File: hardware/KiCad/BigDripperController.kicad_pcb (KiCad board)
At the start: 4 copper layers, 209.1 x 208.6 mm, 95 parts, among them Q1 IRL540NPBF, Q10 IRL540NPBF, Q11 IRL540NPBF, Q12 IRL540NPBF, Q13 IRL540NPBF, Q14 IRL540NPBF, Q15 IRL540NPBF, Q16 IRL540NPBF, Q17 TL2575-05IKV, Q2 IRL540NPBF, Q3 IRL540NPBF, Q4 IRL540NPBF, Q5 IRL540NPBF, Q6 IRL540NPBF, Q7 IRL540NPBF, Q8 IRL540NPBF, Q9 IRL540NPBF, U18 SN74HCT125NE4, U2 SN74HCT125NE4, U3 SN74HCT125NE4, U4 SN74HCT125NE4, U5 SN74HCT125NE4

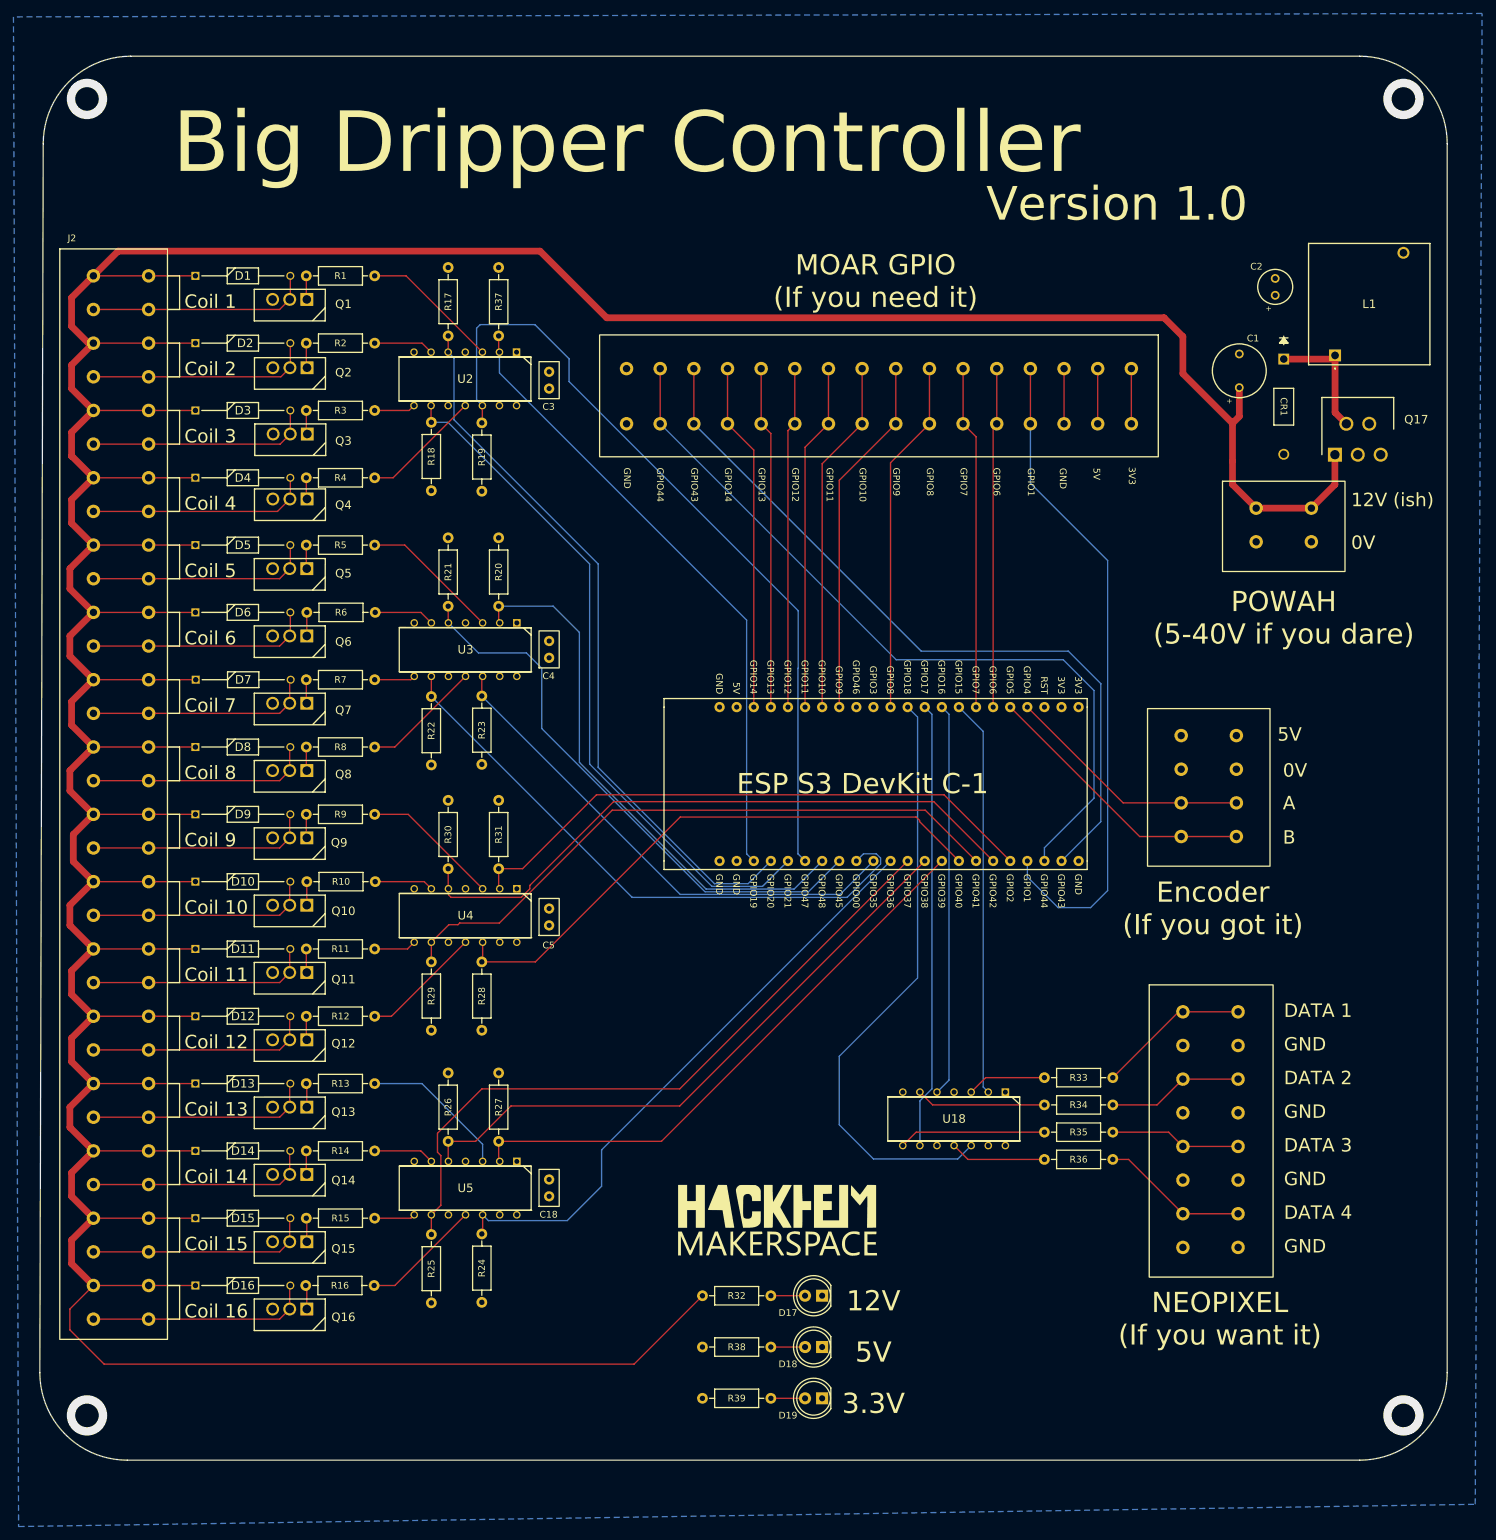
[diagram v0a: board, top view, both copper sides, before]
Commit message: Added updated schematic and layout.
* Added production files for 1.1
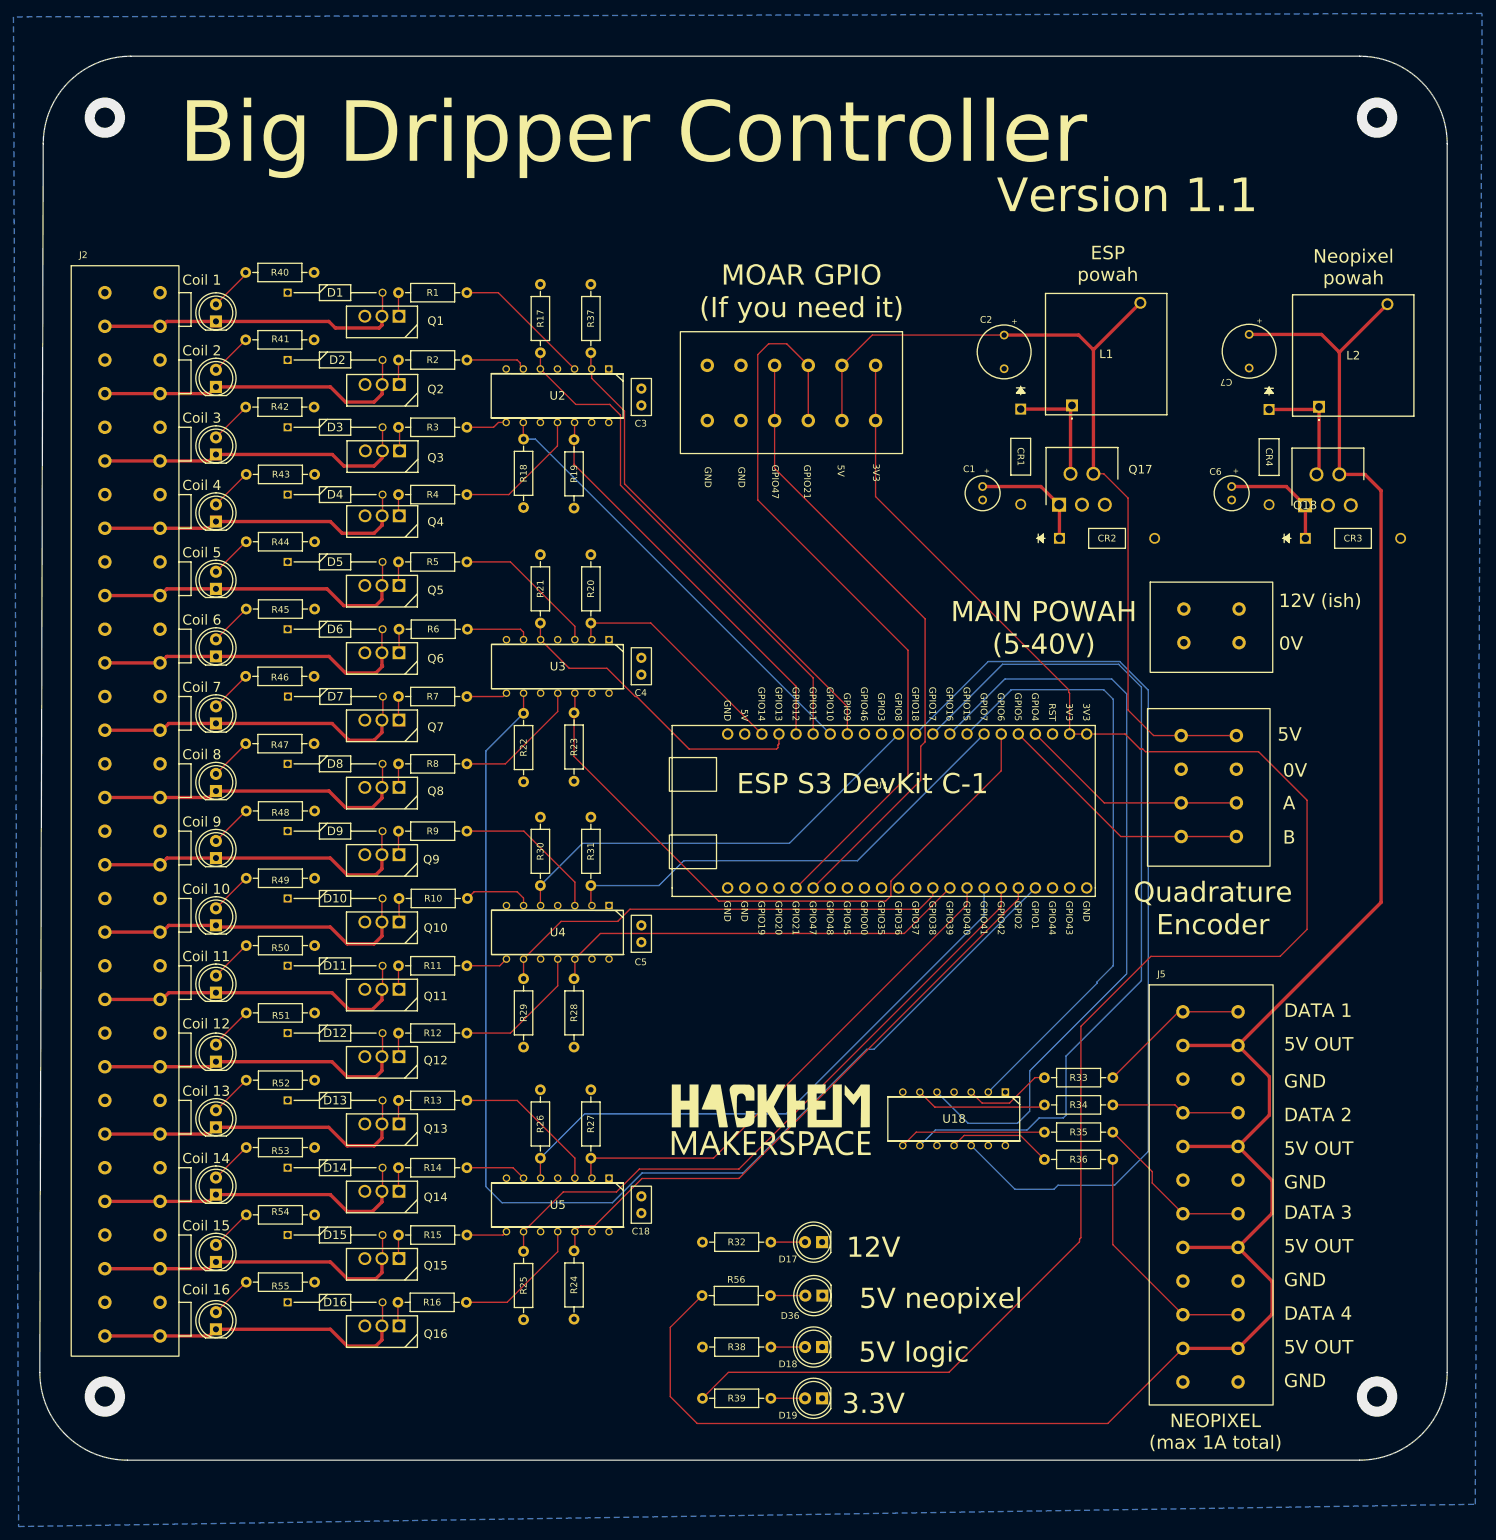
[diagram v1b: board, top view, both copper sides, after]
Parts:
- added C6: 100uF, hackheim:CAP ALUM 10UF 20% 25V RADIAL TH - WÜRTH - 860020472003, F.Cu at (223.4, 40.8)
- added C7: 330uF, hackheim:CAP ALUM 10UF 20% 25V RADIAL TH - WÜRTH - 860020472003, F.Cu at (226.5, 18.2)
- added CR2: 1N5819, hackheim:DO-41_STM, F.Cu at (197.8, 47.5)
- added CR3: 1N5819, hackheim:DO-41_STM, F.Cu at (234.4, 47.5)
- added CR4: 1N5819, hackheim:DO-41_STM, F.Cu at (229.0, 28.4)
- added D20: LED, LED_THT:LED_D5.0mm, F.Cu at (72.5, 15.3)
- added D21: LED, LED_THT:LED_D5.0mm, F.Cu at (72.5, 25.0)
- added D22: LED, LED_THT:LED_D5.0mm, F.Cu at (72.5, 35.0)
- added D23: LED, LED_THT:LED_D5.0mm, F.Cu at (72.5, 45.0)
- added D24: LED, LED_THT:LED_D5.0mm, F.Cu at (72.5, 55.0)
- added D25: LED, LED_THT:LED_D5.0mm, F.Cu at (72.5, 65.0)
- added D26: LED, LED_THT:LED_D5.0mm, F.Cu at (72.5, 75.0)
- added D27: LED, LED_THT:LED_D5.0mm, F.Cu at (72.5, 85.0)
- added D28: LED, LED_THT:LED_D5.0mm, F.Cu at (72.5, 95.0)
- added D29: LED, LED_THT:LED_D5.0mm, F.Cu at (72.5, 105.0)
- added D30: LED, LED_THT:LED_D5.0mm, F.Cu at (72.5, 115.0)
- added D31: LED, LED_THT:LED_D5.0mm, F.Cu at (72.5, 125.2)
- added D32: LED, LED_THT:LED_D5.0mm, F.Cu at (72.5, 135.0)
- added D33: LED, LED_THT:LED_D5.0mm, F.Cu at (72.5, 145.0)
- added D34: LED, LED_THT:LED_D5.0mm, F.Cu at (72.5, 155.0)
- added D35: LED, LED_THT:LED_D5.0mm, F.Cu at (72.5, 165.0)
- added D36: LED, LED_THT:LED_D5.0mm, F.Cu at (162.6, 160.0)
- added L2: PE-52627NL, hackheim:PE52627NL, F.Cu at (236.4, 28.0)
- added Q18: TL2575-05IKV, hackheim:TL2575-05IKV, F.Cu at (234.3, 42.6)
- added R40: 2k, Resistor_THT:R_Axial_DIN0207_L6.3mm_D2.5mm_P10.16mm_Horizontal, F.Cu at (87.1, 8.00)
- added R41: 2k, Resistor_THT:R_Axial_DIN0207_L6.3mm_D2.5mm_P10.16mm_Horizontal, F.Cu at (87.1, 18.0)
- added R42: 2k, Resistor_THT:R_Axial_DIN0207_L6.3mm_D2.5mm_P10.16mm_Horizontal, F.Cu at (87.1, 28.0)
- added R43: 2k, Resistor_THT:R_Axial_DIN0207_L6.3mm_D2.5mm_P10.16mm_Horizontal, F.Cu at (87.2, 38.0)
- added R44: 2k, Resistor_THT:R_Axial_DIN0207_L6.3mm_D2.5mm_P10.16mm_Horizontal, F.Cu at (87.2, 48.0)
- added R45: 2k, Resistor_THT:R_Axial_DIN0207_L6.3mm_D2.5mm_P10.16mm_Horizontal, F.Cu at (87.2, 58.0)
- added R46: 2k, Resistor_THT:R_Axial_DIN0207_L6.3mm_D2.5mm_P10.16mm_Horizontal, F.Cu at (87.1, 68.0)
- added R47: 2k, Resistor_THT:R_Axial_DIN0207_L6.3mm_D2.5mm_P10.16mm_Horizontal, F.Cu at (87.1, 78.0)
- added R48: 2k, Resistor_THT:R_Axial_DIN0207_L6.3mm_D2.5mm_P10.16mm_Horizontal, F.Cu at (87.2, 88.0)
- added R49: 2k, Resistor_THT:R_Axial_DIN0207_L6.3mm_D2.5mm_P10.16mm_Horizontal, F.Cu at (87.2, 98.0)
- added R50: 2k, Resistor_THT:R_Axial_DIN0207_L6.3mm_D2.5mm_P10.16mm_Horizontal, F.Cu at (87.2, 108.0)
- added R51: 2k, Resistor_THT:R_Axial_DIN0207_L6.3mm_D2.5mm_P10.16mm_Horizontal, F.Cu at (87.2, 118.0)
- added R52: 2k, Resistor_THT:R_Axial_DIN0207_L6.3mm_D2.5mm_P10.16mm_Horizontal, F.Cu at (87.2, 128.0)
- added R53: 2k, Resistor_THT:R_Axial_DIN0207_L6.3mm_D2.5mm_P10.16mm_Horizontal, F.Cu at (87.2, 138.0)
- added R54: 2k, Resistor_THT:R_Axial_DIN0207_L6.3mm_D2.5mm_P10.16mm_Horizontal, F.Cu at (87.2, 148.0)
- added R55: 2k, Resistor_THT:R_Axial_DIN0207_L6.3mm_D2.5mm_P10.16mm_Horizontal, F.Cu at (87.2, 158.0)
- added R56: R, Resistor_THT:R_Axial_DIN0207_L6.3mm_D2.5mm_P10.16mm_Horizontal, F.Cu at (144.7, 160.0)
- moved C1 43.4 mm to (186.4, 40.8), turned to 90 degrees
- moved C2 42.7 mm to (188.6, 19.8), turned to 90 degrees
- moved Q17 41.6 mm to (197.8, 42.5)
- moved CR1 39.8 mm to (192.1, 28.3)
- moved L1 39.8 mm to (199.7, 27.8)
- moved J4 38.0 mm to (170.5, 21.8)
- moved J1 18.4 mm to (216.3, 58.0)
- moved REF** 14.9 mm to (154.0, 132.4)
- moved R19 13.9 mm to (125.7, 32.8)
- moved D1 13.9 mm to (83.2, 11.0)
- moved D10 13.9 mm to (83.2, 101.0)
- moved D11 13.9 mm to (83.2, 111.0)
- moved D12 13.9 mm to (83.2, 121.0)
- moved D13 13.9 mm to (83.2, 131.0)
- moved D14 13.9 mm to (83.2, 141.0)
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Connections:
- net Net-(D1-A) renamed C1
- net Net-(D10-A) renamed C10
- net Net-(D11-A) renamed C11
- net Net-(D12-A) renamed C12
- net Net-(D13-A) renamed C13
- net Net-(D14-A) renamed C14
- net Net-(D15-A) renamed C15
- net Net-(D16-A) renamed C16
- net Net-(D2-A) renamed C2
- net Net-(D3-A) renamed C3
- net Net-(D4-A) renamed C4
- net Net-(D5-A) renamed C5
- net Net-(D6-A) renamed C6
- net Net-(D7-A) renamed C7
- net Net-(D8-A) renamed C8
- net Net-(D9-A) renamed C9
- C1 pad 1: 12V -> Net-(Q17-VIN)
- J4 pad 3: GND -> GPIO21
- J4 pad 4: GPIO1 -> GPIO47
- J4 pad 5: GPIO6 -> GND
- J4 pad 6: GPIO7 -> GND
- Q17 pad 1: 12V -> Net-(Q17-VIN)
- U1 pad 12: GPIO8 -> COIL15
- U1 pad 15: GPIO9 -> COIL1
- U1 pad 16: GPIO10 -> COIL3
- U1 pad 17: GPIO11 -> COIL2
- U1 pad 18: GPIO12 -> COIL4
- U1 pad 19: GPIO13 -> COIL6
- U1 pad 20: GPIO14 -> COIL5
- U1 pad 25: COIL1 -> unconnected-(U1-GPIO19-Pad25)
- U1 pad 26: COIL2 -> unconnected-(U1-GPIO20-Pad26)
- U1 pad 27: COIL3 -> GPIO21
- U1 pad 28: COIL4 -> GPIO47
- U1 pad 29: COIL5 -> unconnected-(U1-GPIO48-Pad29)
- U1 pad 30: COIL6 -> unconnected-(U1-GPIO45-Pad30)
- U1 pad 31: COIL7 -> unconnected-(U1-GPIO0-Pad31)
- U1 pad 32: COIL8 -> unconnected-(U1-GPIO35-Pad32)
- U1 pad 33: COIL9 -> unconnected-(U1-GPIO36-Pad33)
- U1 pad 34: COIL10 -> unconnected-(U1-GPIO37-Pad34)
- U1 pad 35: COIL11 -> COIL14
- U1 pad 36: COIL12 -> COIL13
- U1 pad 37: COIL13 -> COIL12
- U1 pad 38: COIL14 -> COIL11
- U1 pad 39: COIL15 -> COIL10
- U1 pad 40: COIL16 -> COIL9
- U1 pad 41: GPIO1 -> COIL7
- U1 pad 42: GPIO44 -> unconnected-(U1-GPIO44-Pad42)
- U1 pad 43: GPIO43 -> unconnected-(U1-GPIO43-Pad43)
- U1 pad 6: GPIO6 -> COIL8
- U1 pad 7: GPIO7 -> COIL16
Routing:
- net 12V: track 764.4 -> 0.00 mm
- net NEOPIXEL_5V: track 0.00 -> 330.6 mm
- net 3V3: track 8.20 -> 262.6 mm
- net 5V: track 8.20 -> 132.4 mm
- net GPIO44: track 117.4 -> 0.00 mm
- net GPIO43: track 113.4 -> 0.00 mm
- net GPIO21: track 0.00 -> 113.0 mm
- net GPIO1: track 99.5 -> 0.00 mm
- net GPIO47: track 0.00 -> 93.8 mm
- net COIL7: track 89.3 -> 177.6 mm
- net NEOPIXEL_3_DATA: track 66.3 -> 128.5 mm
- net COIL4: track 119.7 -> 60.0 mm
- net NEOPIXEL_2_DATA: track 58.4 -> 115.0 mm
- net GPIO9: track 53.8 -> 0.00 mm
- net GPIO10: track 52.7 -> 0.00 mm
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- added copper zone on In1.Cu, net 12V
- added copper zone on B.Cu, net GND
- removed copper zone on B.Cu, net 3V3
- removed copper zone on In1.Cu, net GND
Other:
- board text added: "5V logic"
- board text added: "5V neopixel"
- board text added: "ESP powah"
- board text added: "MAIN POWAH (5-40V)"
- board text added: "NEOPIXEL (max 1A total)"
- board text added: "Neopixel powah"
- board text added: "Quadrature Encoder"
- board text added: "Version 1.1"
- board text removed: "5V"
- board text removed: "Encoder (If you got it)"
- board text removed: "NEOPIXEL (If you want it)"
- board text removed: "POWAH (5-40V if you dare)"
- board text removed: "Version 1.0"
